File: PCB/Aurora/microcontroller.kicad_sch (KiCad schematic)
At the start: 39 parts, among them IC2 STM32G0B1KBU6

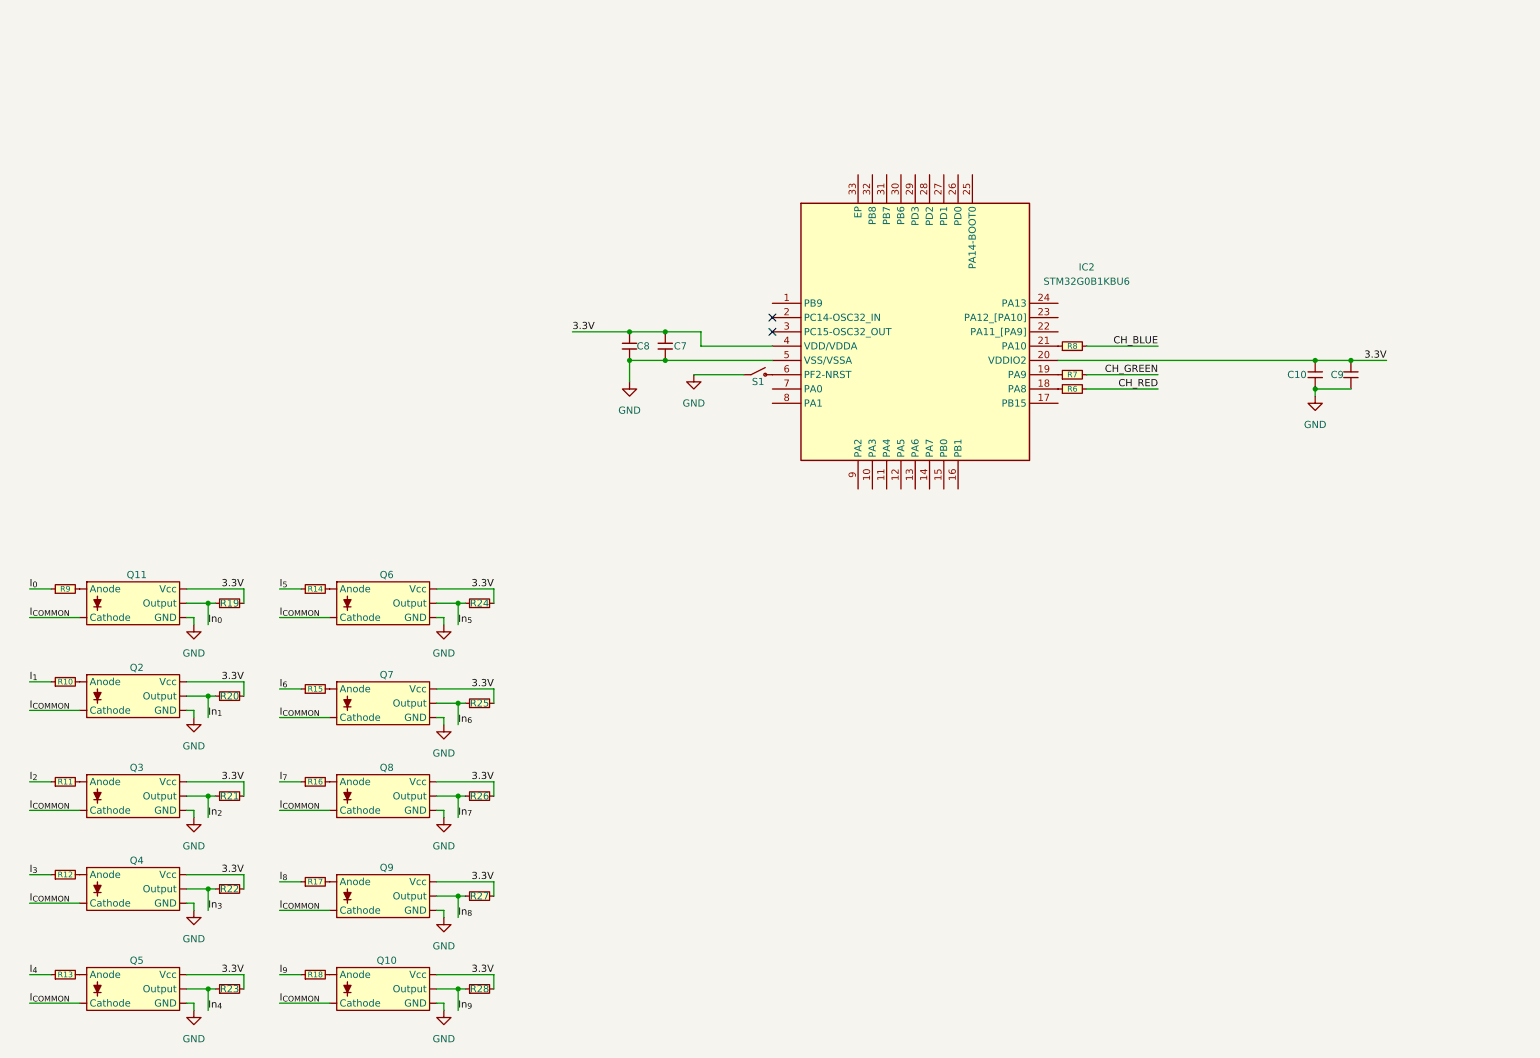
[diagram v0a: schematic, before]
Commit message: Schema + PCB
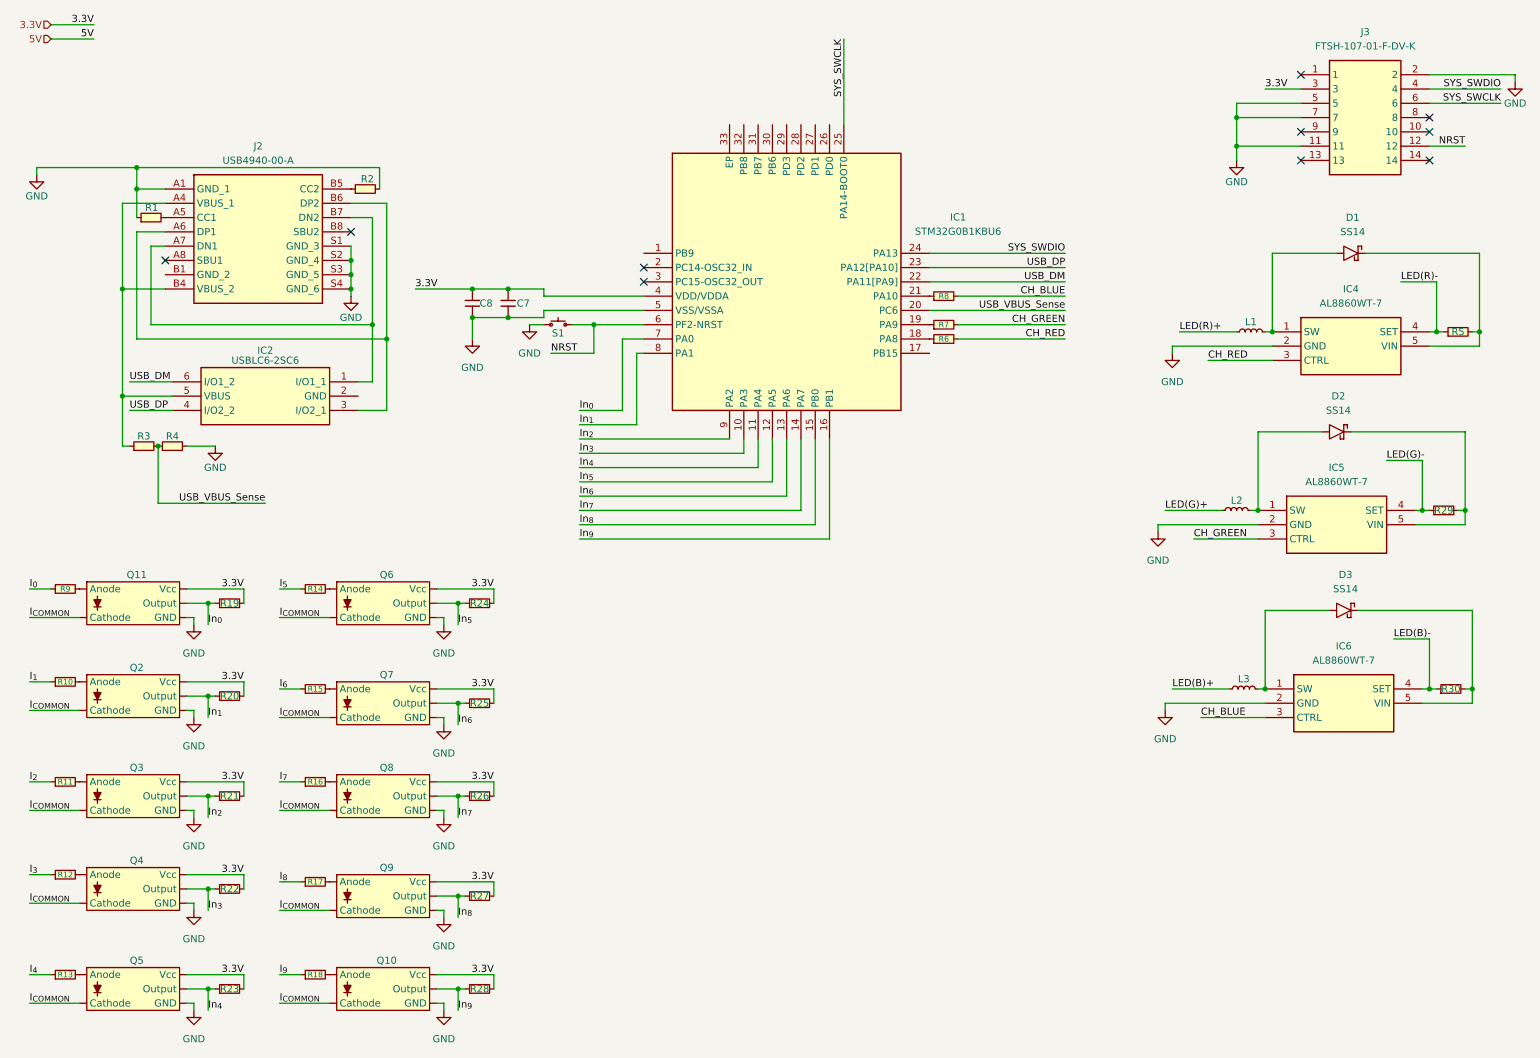
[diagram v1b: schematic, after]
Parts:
- removed C10: 100nF, Capacitor_SMD:C_0402_1005Metric, symbol SamacSys_Parts:AC0402KRX7R7BB104
- removed C9: 4.7uF, SamacSys_Parts:C0402C104J4RACTU, symbol SamacSys_Parts:C0402C475K8PACTU
- removed IC2: STM32G0B1KBU6, QFN50P500X500X60-33N-D, symbol SamacSys_Parts:STM32G0B1KBU6
- added D1, D2, D3: SS14, DIOM5227X270N, symbol SamacSys:SS14
- added IC1: STM32G0B1KBU6, SamacSys:QFN50P500X500X60-33N-D, symbol SamacSys:STM32G0B1KBU6
- added IC2: USBLC6-2SC6, SamacSys:SOT95P280X145-6N, symbol SamacSys:USBLC6-2SC6
- added IC4, IC5, IC6: AL8860WT-7, SOT95P280X100-5N, symbol SamacSys:AL8860WT-7
- added J2: USB4940-00-A, USB494000A, symbol SamacSys:USB4940-00-A
- added J3: FTSH-107-01-F-DV-K, FTSH-107-XX-YYY-DV-K, symbol SamacSys:FTSH-107-01-F-DV-K
- added L1, L2, L3: PA4332.472NLT, PA4332472NLT, symbol SamacSys:PA4332.472NLT
- added R1, R2: CR0603-FX-5101ELF, RESC1608X55N, symbol SamacSys:CR0603-FX-5101ELF
- added R29, R30, R5: 0.16R, Resistor_SMD:R_0603_1608Metric, symbol SamacSys:RL0603FR-070R16L
- added R3: MCT0603MC3302FP500, RESC1608X55N, symbol SamacSys:MCT0603MC3302FP500
- added R4: ERJ-P08F8202V, ERJP08_(1206), symbol SamacSys:ERJ-P08F8202V
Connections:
- net 3.3V: now also IC1.4 (VDD/VDDA), J3.3
- net CH_BLUE: now also IC6.3 (CTRL)
- net CH_GREEN: now also IC5.3 (CTRL)
- net CH_RED: now also IC4.3 (CTRL)
- net GND: now also IC1.5 (VSS/VSSA), IC4.2 (GND), IC5.2 (GND), IC6.2 (GND), J2.A1 (GND_1), J2.S1 (GND_3), J2.S2 (GND_4), J2.S3 (GND_5), J2.S4 (GND_6), J3.11, J3.2, J3.5, J3.7, R1.1, R2.2, R4.2
- net In_{0}: now also IC1.7 (PA0)
- net In_{1}: now also IC1.8 (PA1)
- net In_{2}: now also IC1.9 (PA2)
- net In_{3}: now also IC1.10 (PA3)
- net In_{4}: now also IC1.11 (PA4)
- net In_{5}: now also IC1.12 (PA5)
- net In_{6}: now also IC1.13 (PA6)
- net In_{7}: now also IC1.14 (PA7)
- net In_{8}: now also IC1.15 (PB0)
- net In_{9}: now also IC1.16 (PB1)
- net at R6.1: now also IC1.18 (PA8)
- net at R7.1: now also IC1.19 (PA9)
- net at R8.1: now also IC1.21 (PA10)
- net NRST: now reaches S1.2
- net NRST: now also IC1.6 (PF2-NRST), J3.12
- new net: IC2.1 (I/O1_1), J2.A7 (DN1), J2.B7 (DN2)
- new net: IC2.3 (I/O2_1), J2.A6 (DP1), J2.B6 (DP2)
- new net: IC2.5 (VBUS), J2.A4 (VBUS_1), J2.B4 (VBUS_2), R3.1
- new net: D3.2, IC6.1 (SW), L3.2
- new net: J2.A5 (CC1), R1.2
- new net: J2.B5 (CC2), R2.1
- new net: D2.1, IC5.5 (VIN), R29.2
- new net: D2.2, IC5.1 (SW), L2.2
- new net: D3.1, IC6.5 (VIN), R30.2
- new net: D1.2, IC4.1 (SW), L1.2
- new net: D1.1, IC4.5 (VIN), R5.2
- new net LED(B)+: L3.1
- new net LED(B)-: IC6.4 (SET), R30.1
- new net LED(G)+: L2.1
- new net LED(G)-: IC5.4 (SET), R29.1
- new net LED(R)+: L1.1
- new net LED(R)-: IC4.4 (SET), R5.1
- new net SYS_SWCLK: IC1.25 (PA14-BOOT0), J3.6
- new net SYS_SWDIO: IC1.24 (PA13), J3.4
- new net USB_DM: IC1.22 (PA11[PA9]), IC2.6 (I/O1_2)
- new net USB_DP: IC1.23 (PA12[PA10]), IC2.4 (I/O2_2)
- new net USB_VBUS_Sense: IC1.20 (PC6), R3.2, R4.1
- no-connect marks 2 -> 10
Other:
- moved on the sheet: C7, C8, R6, R7, R8
